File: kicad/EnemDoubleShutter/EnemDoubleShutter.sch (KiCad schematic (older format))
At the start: 7 parts, among them J1 Conn_01x02, J2 Bouton 1, J3 Bouton 2, U1 NodeMCU_Amica_R2

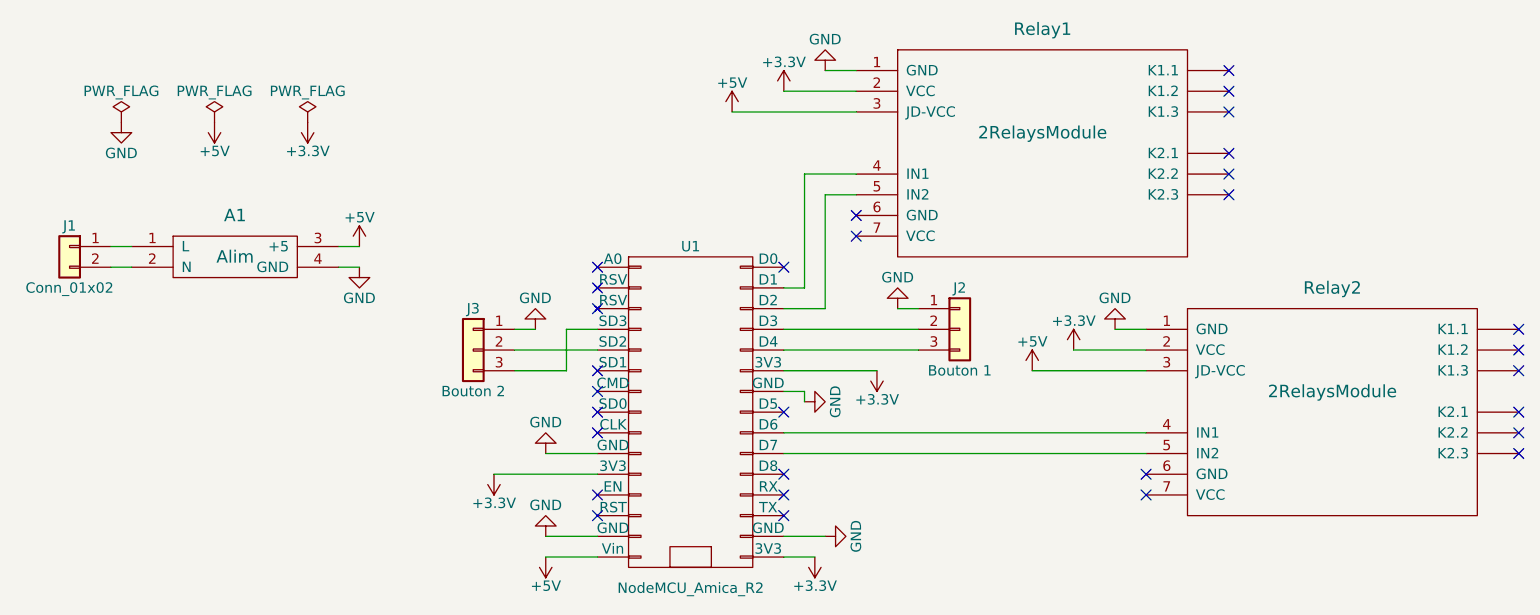
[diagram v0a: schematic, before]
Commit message: Corrections et finalisation PCB
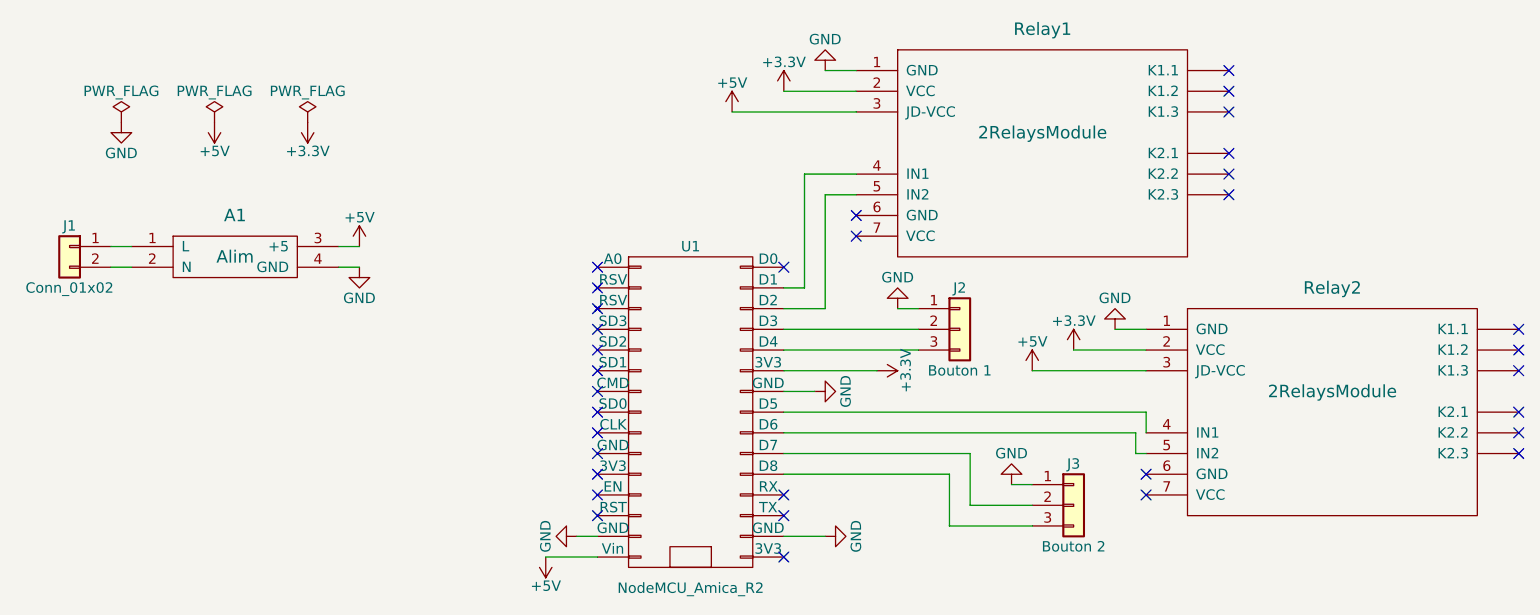
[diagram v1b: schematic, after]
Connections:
- net +3V3: no longer U1.11 (3V3), U1.16 (3V3)
- net GND: no longer U1.10 (GND)
- net at U1.20 (D8): now also J3.3 (Pin_3)
- net at U1.21 (D7): now also J3.2 (Pin_2); no longer Relay2.5 (IN2)
- net at U1.22 (D6): now also Relay2.5 (IN2); no longer Relay2.4 (IN1)
- net at U1.23 (D5): now also Relay2.4 (IN1)
- net at U1.4 (SD3): no longer J3.3 (Pin_3)
- net at U1.5 (SD2): no longer J3.2 (Pin_2)
- no-connect marks 30 -> 33
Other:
- moved on the sheet: J3
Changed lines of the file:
@@
 LIBS:contrib
 LIBS:valves
+LIBS:enem
 LIBS:nodemcu
-LIBS:enem
 LIBS:EnemDoubleShutter-cache
 EELAYER 25 0
@@
 $EndDescr
 $Comp
-L GND #PWR01
-U 1 1 5AE0C572
-P 4650 4750
-F 0 "#PWR01" H 4650 4500 50  0001 C CNN
-F 1 "GND" H 4650 4600 50  0000 C CNN
-F 2 "" H 4650 4750 50  0001 C CNN
-F 3 "" H 4650 4750 50  0001 C CNN
-	1    4650 4750
-	-1   0    0    1
-$EndComp
-$Comp
-L +5V #PWR02
+L +5V #PWR01
 U 1 1 5AE34FA2
 P 4650 4850
-F 0 "#PWR02" H 4650 4700 50  0001 C CNN
+F 0 "#PWR01" H 4650 4700 50  0001 C CNN
 F 1 "+5V" H 4650 4990 50  0000 C CNN
 F 2 "" H 4650 4850 50  0001 C CNN
@@
 NoConn ~ 5800 4650
 $Comp
-L PWR_FLAG #FLG03
+L PWR_FLAG #FLG02
 U 1 1 5AE354EB
 P 2600 2750
-F 0 "#FLG03" H 2600 2825 50  0001 C CNN
+F 0 "#FLG02" H 2600 2825 50  0001 C CNN
 F 1 "PWR_FLAG" H 2600 2900 50  0000 C CNN
 F 2 "" H 2600 2750 50  0001 C CNN
@@
 $EndComp
 $Comp
-L PWR_FLAG #FLG04
+L PWR_FLAG #FLG03
 U 1 1 5AE35505
 P 3050 2750
-F 0 "#FLG04" H 3050 2825 50  0001 C CNN
+F 0 "#FLG03" H 3050 2825 50  0001 C CNN
 F 1 "PWR_FLAG" H 3050 2900 50  0000 C CNN
 F 2 "" H 3050 2750 50  0001 C CNN
@@
 $EndComp
 $Comp
-L GND #PWR05
+L GND #PWR04
 U 1 1 5AE3551F
 P 2600 2750
-F 0 "#PWR05" H 2600 2500 50  0001 C CNN
+F 0 "#PWR04" H 2600 2500 50  0001 C CNN
 F 1 "GND" H 2600 2600 50  0000 C CNN
 F 2 "" H 2600 2750 50  0001 C CNN
@@
 $EndComp
 $Comp
-L +5V #PWR06
+L +5V #PWR05
 U 1 1 5AE35537
 P 3050 2750
-F 0 "#PWR06" H 3050 2600 50  0001 C CNN
+F 0 "#PWR05" H 3050 2600 50  0001 C CNN
 F 1 "+5V" H 3050 2890 50  0000 C CNN
 F 2 "" H 3050 2750 50  0001 C CNN
@@
 $EndComp
 $Comp
-L GND #PWR07
+L GND #PWR06
 U 1 1 5AE62183
 P 3750 3450
-F 0 "#PWR07" H 3750 3200 50  0001 C CNN
+F 0 "#PWR06" H 3750 3200 50  0001 C CNN
 F 1 "GND" H 3750 3300 50  0000 C CNN
 F 2 "" H 3750 3450 50  0001 C CNN
@@
 $EndComp
 $Comp
-L +5V #PWR08
+L +5V #PWR07
 U 1 1 5AE6219F
 P 3750 3350
-F 0 "#PWR08" H 3750 3200 50  0001 C CNN
+F 0 "#PWR07" H 3750 3200 50  0001 C CNN
 F 1 "+5V" H 3750 3490 50  0000 C CNN
 F 2 "" H 3750 3350 50  0001 C CNN
@@
 $EndComp
 $Comp
-L GND #PWR09
+L GND #PWR08
 U 1 1 5AE629DE
 P 6000 2500
-F 0 "#PWR09" H 6000 2250 50  0001 C CNN
+F 0 "#PWR08" H 6000 2250 50  0001 C CNN
 F 1 "GND" H 6000 2350 50  0000 C CNN
 F 2 "" H 6000 2500 50  0001 C CNN
@@
 $EndComp
 $Comp
-L +3.3V #PWR010
-U 1 1 5AE62AB6
-P 5950 4850
-F 0 "#PWR010" H 5950 4700 50  0001 C CNN
-F 1 "+3.3V" H 5950 4990 50  0000 C CNN
-F 2 "" H 5950 4850 50  0001 C CNN
-F 3 "" H 5950 4850 50  0001 C CNN
-	1    5950 4850
-	-1   0    0    1
-$EndComp
-$Comp
-L +3.3V #PWR011
+L +3.3V #PWR09
 U 1 1 5AE62AFA
 P 3500 2750
-F 0 "#PWR011" H 3500 2600 50  0001 C CNN
+F 0 "#PWR09" H 3500 2600 50  0001 C CNN
 F 1 "+3.3V" H 3500 2890 50  0000 C CNN
 F 2 "" H 3500 2750 50  0001 C CNN
@@
 $EndComp
 $Comp
-L PWR_FLAG #FLG012
+L PWR_FLAG #FLG010
 U 1 1 5AE62B41
 P 3500 2750
-F 0 "#FLG012" H 3500 2825 50  0001 C CNN
+F 0 "#FLG010" H 3500 2825 50  0001 C CNN
 F 1 "PWR_FLAG" H 3500 2900 50  0000 C CNN
 F 2 "" H 3500 2750 50  0001 C CNN
@@
 $EndComp
 $Comp
-L +3.3V #PWR013
+L +3.3V #PWR011
 U 1 1 5AE62B99
 P 5800 2600
-F 0 "#PWR013" H 5800 2450 50  0001 C CNN
+F 0 "#PWR011" H 5800 2450 50  0001 C CNN
 F 1 "+3.3V" H 5800 2740 50  0000 C CNN
 F 2 "" H 5800 2600 50  0001 C CNN
@@
 $EndComp
 $Comp
-L +5V #PWR014
+L +5V #PWR012
 U 1 1 5AE62BE5
 P 5550 2700
-F 0 "#PWR014" H 5550 2550 50  0001 C CNN
+F 0 "#PWR012" H 5550 2550 50  0001 C CNN
 F 1 "+5V" H 5550 2840 50  0000 C CNN
 F 2 "" H 5550 2700 50  0001 C CNN
@@
 $EndComp
 $Comp
-L GND #PWR015
+L GND #PWR013
 U 1 1 5AE6306B
 P 6350 3650
-F 0 "#PWR015" H 6350 3400 50  0001 C CNN
+F 0 "#PWR013" H 6350 3400 50  0001 C CNN
 F 1 "GND" H 6350 3500 50  0000 C CNN
 F 2 "" H 6350 3650 50  0001 C CNN
@@
 $EndComp
 $Comp
-L GND #PWR016
+L GND #PWR014
 U 1 1 5AE8BBDB
 P 7400 3750
-F 0 "#PWR016" H 7400 3500 50  0001 C CNN
+F 0 "#PWR014" H 7400 3500 50  0001 C CNN
 F 1 "GND" H 7400 3600 50  0000 C CNN
 F 2 "" H 7400 3750 50  0001 C CNN
@@
 $EndComp
 $Comp
-L +3.3V #PWR017
+L +3.3V #PWR015
 U 1 1 5AE8BBF8
 P 7200 3850
-F 0 "#PWR017" H 7200 3700 50  0001 C CNN
+F 0 "#PWR015" H 7200 3700 50  0001 C CNN
 F 1 "+3.3V" H 7200 3990 50  0000 C CNN
 F 2 "" H 7200 3850 50  0001 C CNN
@@
 $EndComp
 $Comp
-L +5V #PWR018
+L +5V #PWR016
 U 1 1 5AE8BC15
 P 7000 3950
-F 0 "#PWR018" H 7000 3800 50  0001 C CNN
+F 0 "#PWR016" H 7000 3800 50  0001 C CNN
 F 1 "+5V" H 7000 4090 50  0000 C CNN
 F 2 "" H 7000 3950 50  0001 C CNN
@@
 L Conn_01x03 J3
 U 1 1 5AE8C308
-P 4300 3850
-F 0 "J3" H 4300 4050 50  0000 C CNN
-F 1 "Bouton 2" H 4300 3650 50  0000 C CNN
-F 2 "enemLib:Bornier3" H 4300 3850 50  0001 C CNN
-F 3 "" H 4300 3850 50  0001 C CNN
-	1    4300 3850
-	-1   0    0    -1
-$EndComp
-$Comp
-L GND #PWR019
+P 7200 4600
+F 0 "J3" H 7200 4800 50  0000 C CNN
+F 1 "Bouton 2" H 7200 4400 50  0000 C CNN
+F 2 "enemLib:Bornier3" H 7200 4600 50  0001 C CNN
+F 3 "" H 7200 4600 50  0001 C CNN
+	1    7200 4600
+	1    0    0    -1
+$EndComp
+$Comp
+L GND #PWR017
 U 1 1 5AE8C3D5
-P 4600 3750
-F 0 "#PWR019" H 4600 3500 50  0001 C CNN
-F 1 "GND" H 4600 3600 50  0000 C CNN
-F 2 "" H 4600 3750 50  0001 C CNN
-F 3 "" H 4600 3750 50  0001 C CNN
-	1    4600 3750
-	1    0    0    1
-$EndComp
-NoConn ~ 5800 4150
+P 6900 4500
+F 0 "#PWR017" H 6900 4250 50  0001 C CNN
+F 1 "GND" H 6900 4350 50  0000 C CNN
+F 2 "" H 6900 4500 50  0001 C CNN
+F 3 "" H 6900 4500 50  0001 C CNN
+	1    6900 4500
+	-1   0    0    1
+$EndComp
 $Comp
 L NodeMCU_Amica_R2 U1
@@
 $EndComp
 NoConn ~ 4900 3950
-NoConn ~ 5800 4450
-$Comp
-L +3.3V #PWR020
-U 1 1 5AE8D74B
-P 4400 4450
-F 0 "#PWR020" H 4400 4300 50  0001 C CNN
-F 1 "+3.3V" H 4400 4590 50  0000 C CNN
-F 2 "" H 4400 4450 50  0001 C CNN
-F 3 "" H 4400 4450 50  0001 C CNN
-	1    4400 4450
-	-1   0    0    1
-$EndComp
-$Comp
-L GND #PWR021
-U 1 1 5AE8D72B
-P 4650 4350
-F 0 "#PWR021" H 4650 4100 50  0001 C CNN
-F 1 "GND" H 4650 4200 50  0000 C CNN
-F 2 "" H 4650 4350 50  0001 C CNN
-F 3 "" H 4650 4350 50  0001 C CNN
-	1    4650 4350
-	-1   0    0    1
-$EndComp
-Wire Wire Line
-	4650 4750 4900 4750
 Wire Wire Line
 	2550 3350 2650 3350
@@
 	4900 4850 4650 4850
 Wire Wire Line
-	5800 4850 5950 4850
-Wire Wire Line
 	6000 2500 6150 2500
 Wire Wire Line
@@
 	6000 3650 5800 3650
 Wire Wire Line
-	7550 4250 5800 4250
-Wire Wire Line
-	5800 4350 7550 4350
-Wire Wire Line
-	4600 3750 4500 3750
-Wire Wire Line
-	4500 3850 4900 3850
-Wire Wire Line
-	4500 3950 4750 3950
-Wire Wire Line
-	4750 3950 4750 3750
-Wire Wire Line
-	4750 3750 4900 3750
-Wire Wire Line
-	4900 4350 4650 4350
-Wire Wire Line
-	4900 4450 4400 4450
-$Comp
-L GND #PWR022
+	6900 4500 7000 4500
+$Comp
+L GND #PWR018
 U 1 1 5AE8D865
-P 5900 4100
-F 0 "#PWR022" H 5900 3850 50  0001 C CNN
-F 1 "GND" H 5900 3950 50  0000 C CNN
-F 2 "" H 5900 4100 50  0001 C CNN
-F 3 "" H 5900 4100 50  0001 C CNN
-	1    5900 4100
+P 5950 4050
+F 0 "#PWR018" H 5950 3800 50  0001 C CNN
+F 1 "GND" H 5950 3900 50  0000 C CNN
+F 2 "" H 5950 4050 50  0001 C CNN
+F 3 "" H 5950 4050 50  0001 C CNN
+	1    5950 4050
 	0    -1   -1   0
 $EndComp
 $Comp
-L +3.3V #PWR023
+L +3.3V #PWR019
 U 1 1 5AE8D885
 P 6250 3950
-F 0 "#PWR023" H 6250 3800 50  0001 C CNN
+F 0 "#PWR019" H 6250 3800 50  0001 C CNN
 F 1 "+3.3V" H 6250 4090 50  0000 C CNN
 F 2 "" H 6250 3950 50  0001 C CNN
 F 3 "" H 6250 3950 50  0001 C CNN
 	1    6250 3950
-	-1   0    0    1
-$EndComp
-$Comp
-L GND #PWR024
+	0    1    1    0
+$EndComp
+$Comp
+L GND #PWR020
 U 1 1 5AE8D8A5
 P 6000 4750
-F 0 "#PWR024" H 6000 4500 50  0001 C CNN
+F 0 "#PWR020" H 6000 4500 50  0001 C CNN
 F 1 "GND" H 6000 4600 50  0000 C CNN
 F 2 "" H 6000 4750 50  0001 C CNN
@@
 $EndComp
 Wire Wire Line
-	5800 4050 5900 4050
-Wire Wire Line
-	5900 4050 5900 4100
-Wire Wire Line
 	5800 3950 6250 3950
 Wire Wire Line
@@
 NoConn ~ 7550 4450
 NoConn ~ 7550 4550
+NoConn ~ 4900 3750
+NoConn ~ 4900 3850
+Wire Wire Line
+	5800 4050 5950 4050
+Wire Wire Line
+	5800 4150 7550 4150
+Wire Wire Line
+	7550 4150 7550 4250
+Wire Wire Line
+	5800 4250 7500 4250
+Wire Wire Line
+	7500 4250 7500 4350
+Wire Wire Line
+	7500 4350 7550 4350
+Wire Wire Line
+	5800 4350 6700 4350
+Wire Wire Line
+	6700 4350 6700 4600
+Wire Wire Line
+	6700 4600 7000 4600
+Wire Wire Line
+	5800 4450 6600 4450
+Wire Wire Line
+	6600 4450 6600 4700
+Wire Wire Line
+	6600 4700 7000 4700
+NoConn ~ 4900 4350
+NoConn ~ 4900 4450
+$Comp
+L GND #PWR021
+U 1 1 5AEF0CFA
+P 4800 4750
+F 0 "#PWR021" H 4800 4500 50  0001 C CNN
+F 1 "GND" H 4800 4600 50  0000 C CNN
+F 2 "" H 4800 4750 50  0001 C CNN
+F 3 "" H 4800 4750 50  0001 C CNN
+	1    4800 4750
+	0    1    1    0
+$EndComp
+Wire Wire Line
+	4800 4750 4900 4750
+NoConn ~ 5800 4850
 $EndSCHEMATC
